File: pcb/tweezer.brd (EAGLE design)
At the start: 20 x 26 mm, 33 parts, among them IC1 AD7995, IC2 TS507CLT, IC3 TS507CLT, IC5 ESDA6V1SC5, IC6 AT24CS04-SOT23

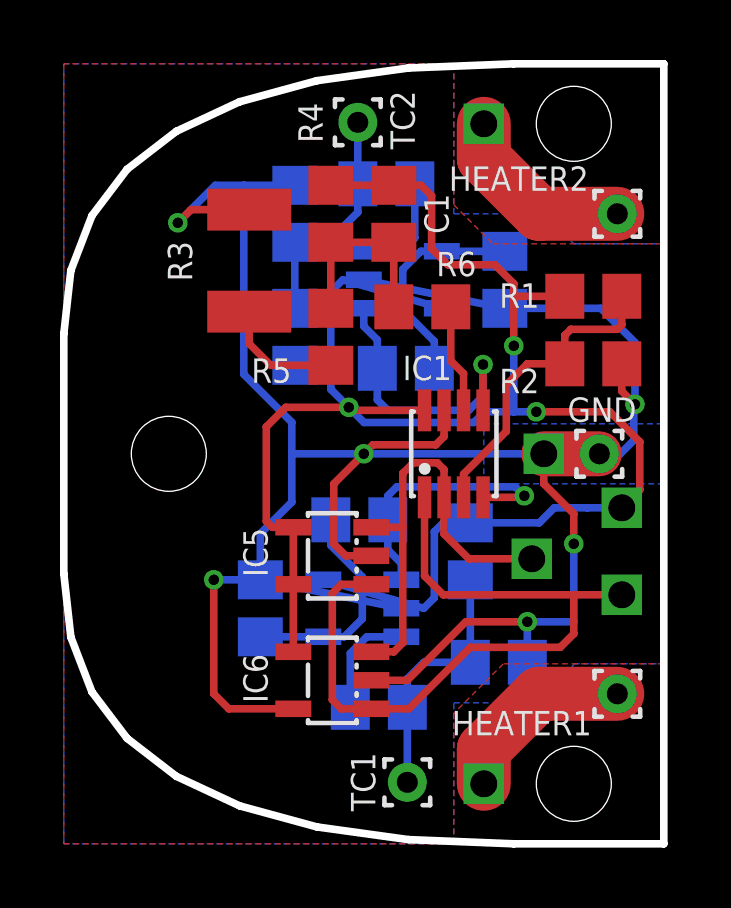
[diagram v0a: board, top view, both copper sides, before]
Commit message: parts reworked
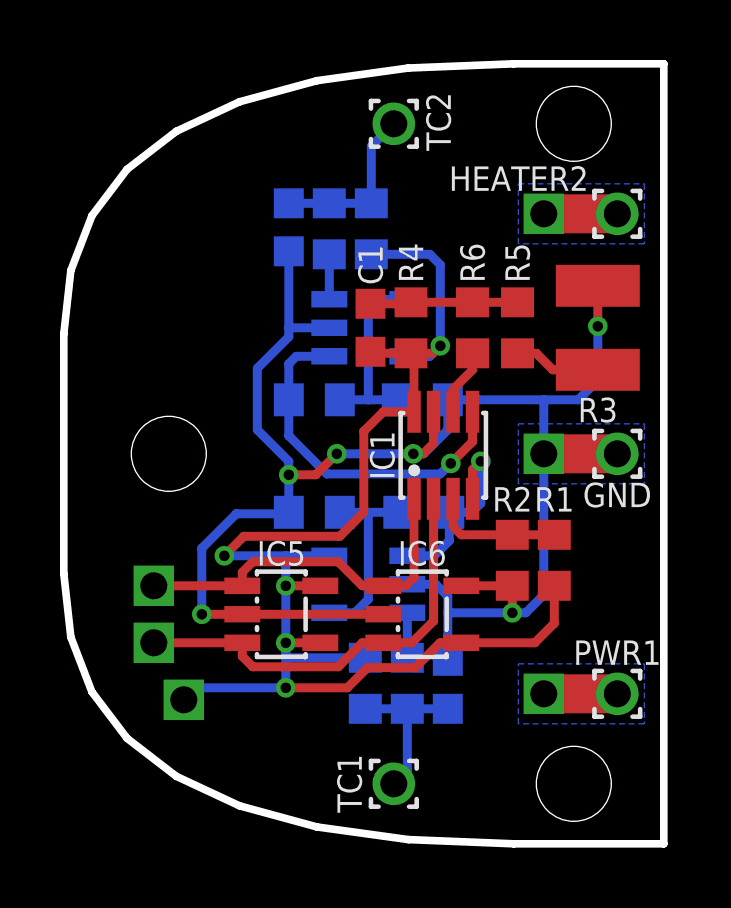
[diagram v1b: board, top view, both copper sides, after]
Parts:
- C1: value 100n -> 100pF; device rcl:C0805 -> common:C0603
- C2, C3: value (none) -> 10nF; device rcl:C0805 -> common:C0603
- R1: value (none) -> 20k 0,1%; device rcl:R0805 -> common:R0603
- R10, R11, R12, R13, R14, R6, R7, R8, R9: device rcl:R0805 -> common:R0603
- R2: value 330k @25°C, 1%, ß=3930 -> 68k @25°C, 1%, ß=3985 K; device solderpi:R0805 -> common:R0603
- R4: value 200k -> 5,1M; device rcl:R0805 -> common:R0603
- R5: value 100k -> 1k; device rcl:R0805 -> common:R0603
- moved U$10 15.9 mm to (4.00, 4.80)
- moved 21 15.6 mm to (3.00, 8.60)
- moved U$9 12.9 mm to (3.00, 6.70)
- moved R3 11.8 mm to (17.8, 17.2)
- moved R1 8.90 mm to (16.4, 9.45), turned to 270 degrees
- moved R2 7.08 mm to (14.9, 9.45), turned to 90 degrees
- moved R5 6.23 mm to (15.1, 17.2)
- moved R9 5.62 mm to (10.1, 5.35)
- moved R14 4.85 mm to (11.9, 14.8), turned to 0 degrees
- moved R4 4.65 mm to (11.6, 17.2), turned to 270 degrees
- moved R13 4.41 mm to (10.2, 20.5)
- moved C1 3.88 mm to (10.2, 17.2), turned to 90 degrees
- moved IC6 3.72 mm to (11.9, 7.65), turned to 270 degrees
- moved R10 3.67 mm to (8.35, 11.1), turned to 180 degrees
- moved U$7 3.61 mm to (16.0, 21.0)
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- renumbered HEATER1 to PWR1
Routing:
- net GND: track 83.9 -> 58.4 mm
- net +5V: track 63.3 -> 48.7 mm, vias 3 -> 5
- net SCL: track 24.9 -> 12.3 mm
- net AD_COMP: track 10.5 -> 4.41 mm
- net HEATER_1: track 6.37 -> 2.45 mm
- net HEATER_2: track 6.37 -> 2.45 mm
- net TC_1: track 8.53 -> 5.44 mm
- net AD_TC_1: track 9.18 -> 6.50 mm
- net AD_TC_2: track 9.68 -> 11.9 mm
- net THERMO_FIL_TC_1: track 3.73 -> 1.50 mm
- net THERMO_FIL1: track 3.69 -> 1.50 mm
- net TC_2: track 7.71 -> 5.71 mm
- net MOTION_FIL: track 6.49 -> 4.92 mm
- net AD_MOTION: track 3.63 -> 2.22 mm
- net MOTION_DIV: track 4.09 -> 2.90 mm
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- added copper zone on layer 1, net GND
- removed copper zone on layer 1, net +5V
- removed copper zone on layer 1, net HEATER_1
- removed copper zone on layer 1, net HEATER_2
